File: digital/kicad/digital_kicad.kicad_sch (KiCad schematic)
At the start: 25 parts, among them J1 Conn_01x01_Pin, J2 Conn_01x01_Pin, J3 Conn_01x01_Pin, J4 Conn_01x01_Pin, Q1 2N3904, Q2 2N3904, Q3 FDN340P, Q4 2N3904, SW1 SW_SPST

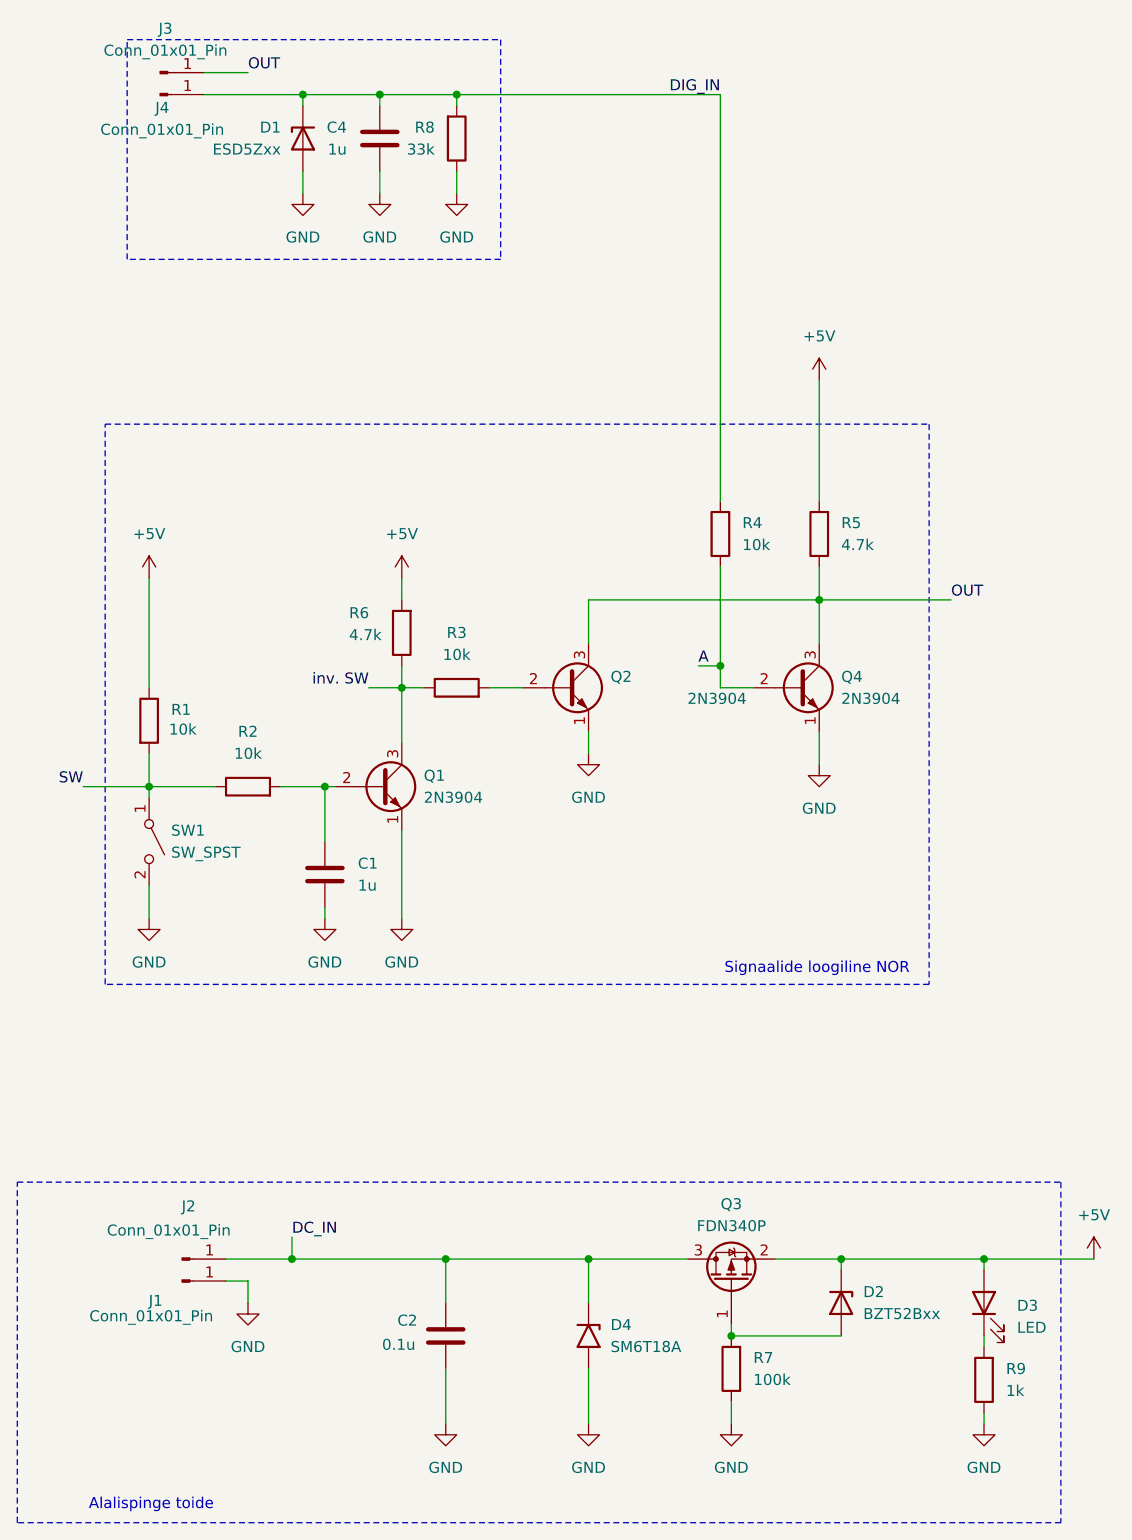
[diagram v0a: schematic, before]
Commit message: sync latest adjustments for final presentation
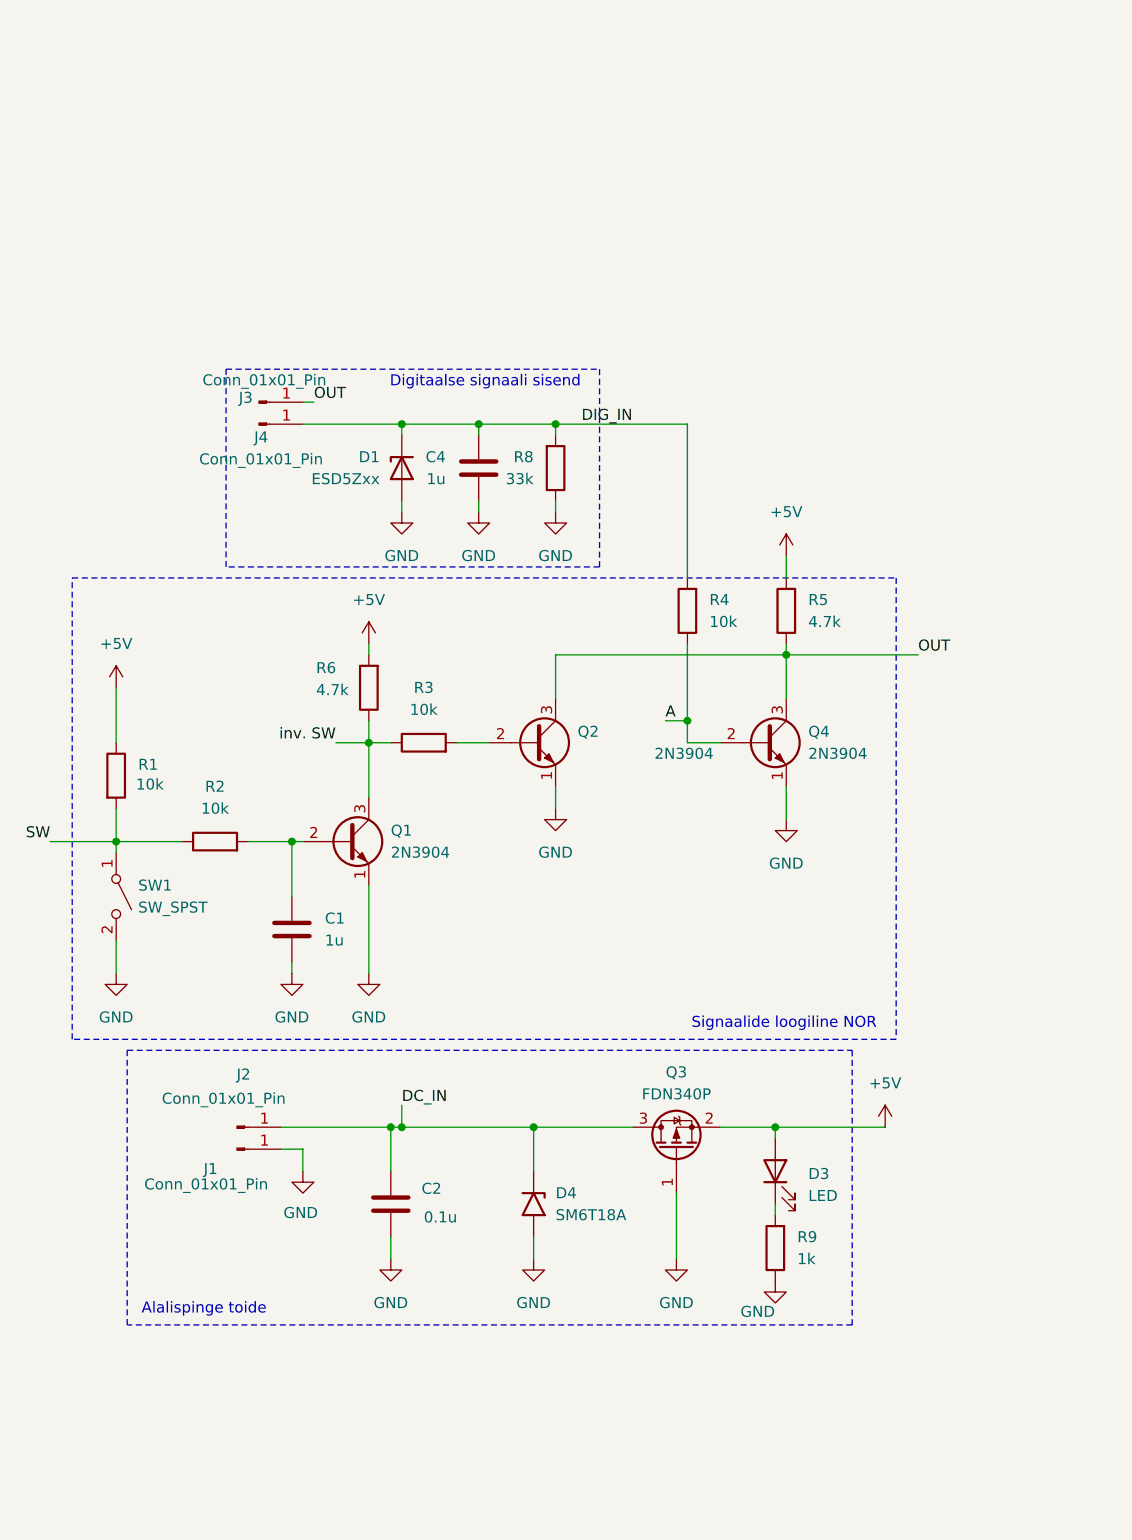
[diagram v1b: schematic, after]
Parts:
- removed D2: BZT52Bxx, Diode_SMD:D_SOD-123F, symbol Diode:BZT52Bxx
- removed R7: 100k, Resistor_SMD:R_0805_2012Metric_Pad1.20x1.40mm_HandSolder, symbol Device:R
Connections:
- net GND: now also Q3.1 (G)
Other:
- note added: "Digitaalse signaali sisend"
- title: (none) -> Arduino digisisendi laiend
- moved on the sheet: C1, C2, C4, D1, D3, D4, J1, J2, J3, J4, Q1, Q2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
